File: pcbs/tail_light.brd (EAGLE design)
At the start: 36 x 20 mm, 13 parts, among them J1 22-27-2041-04

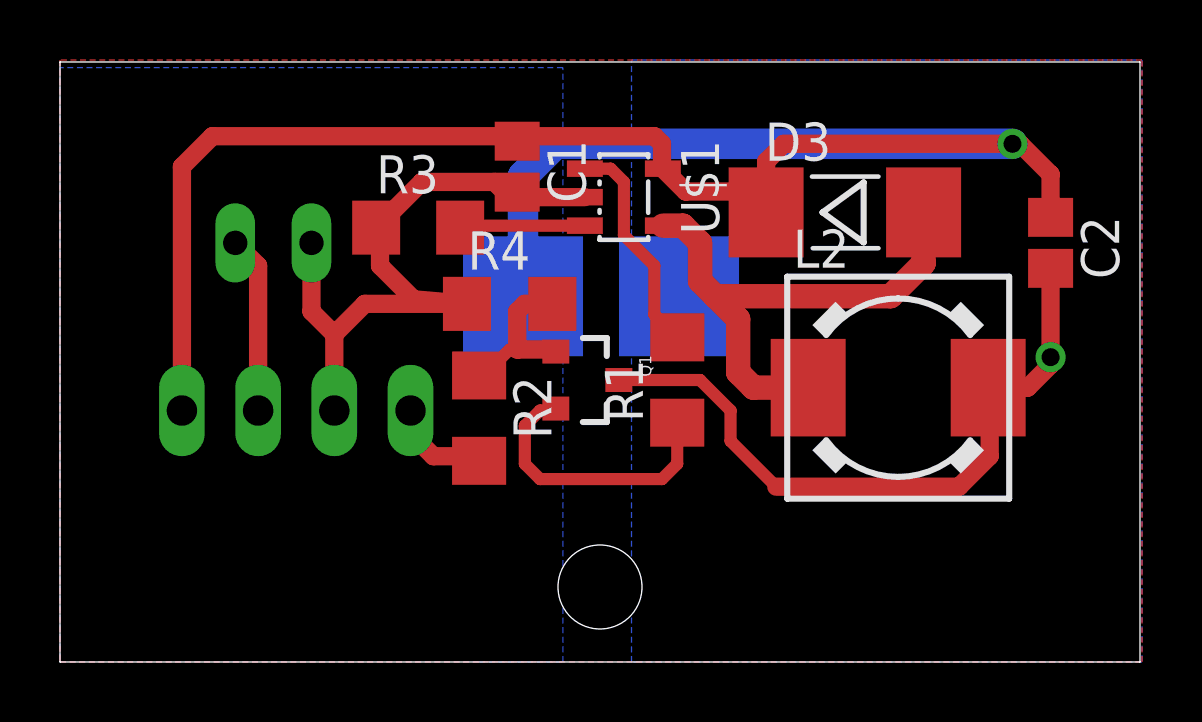
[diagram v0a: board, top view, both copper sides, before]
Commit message: Pcbs: latest changes
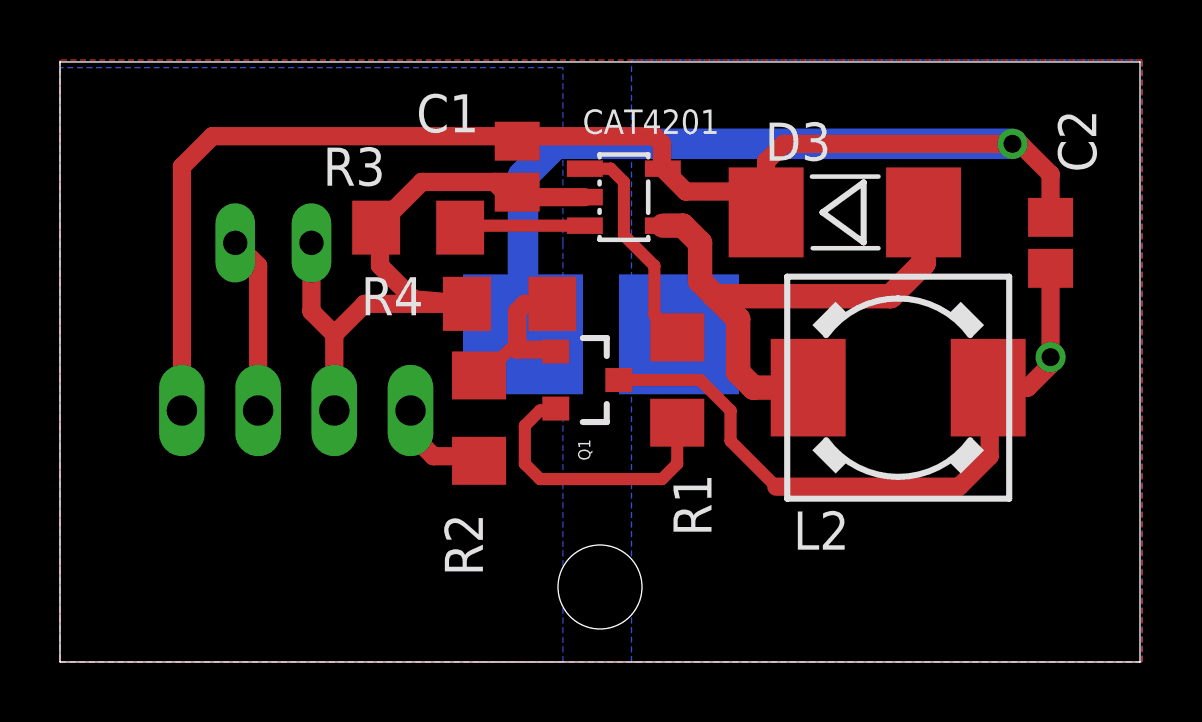
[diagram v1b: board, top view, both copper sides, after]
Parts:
- removed LED1: (no value), led:OSRAM-MINI-TOP-LED
- added LED: (no value), led:OSRAM-MINI-TOP-LED
- renumbered U$1 to CAT4201
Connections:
- net LED_C: now also LED.C; no longer LED1.C
- net VCC: now also LED.A; no longer LED1.A
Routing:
- net VCC: track 64.1 -> 65.3 mm
